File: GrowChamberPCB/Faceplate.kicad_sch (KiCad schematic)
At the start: 56 parts, among them J1 Mister, J10 FoggerBasin, J12 Moisture Sensor 3, J13 Moisture Sensor 2, J14 UART, J15 FAE Fan, J16 DrainLevel, J2 Moisture Sensor 1, J3 SCD30, J4 Heater Fans, J49 TP, J5 Fogger Solenoid, J50 TP, J6 Drain Solenoid, J7 Water Solenoid, J8 Glycol Solenoid, J9 CircFan, SW2 ResetButton_External, SW4 BootMode_External, U2 ZX-IDC2.54-2-13PZZ, U20 PCA9555APW,118

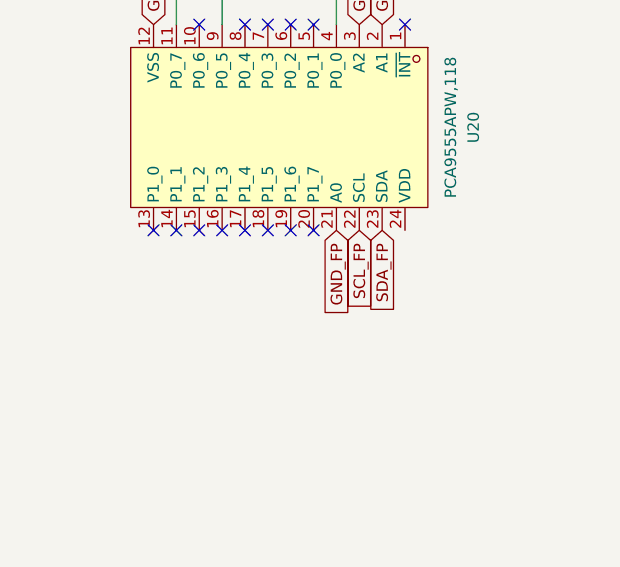
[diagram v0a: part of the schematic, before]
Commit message: working on pcb
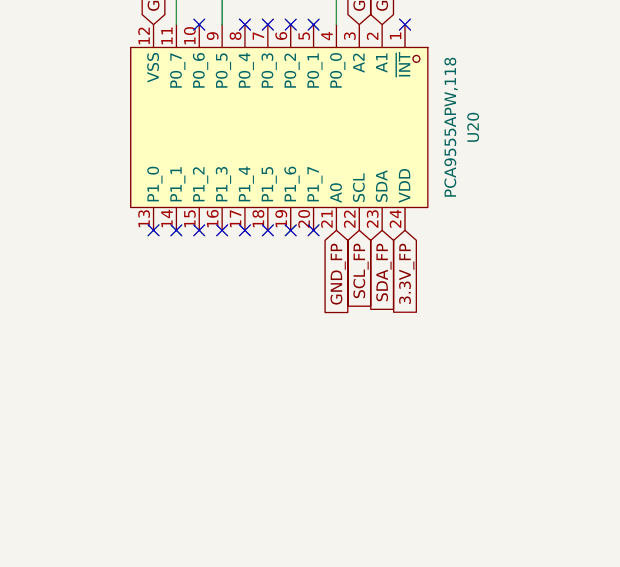
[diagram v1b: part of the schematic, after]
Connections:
- net 3.3V_FP: now also U20.24 (VDD)
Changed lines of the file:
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@@
+		)
+	)
+	(global_label "3.3V_FP"
+		(shape input)
+		(at 265.43 139.7 270)
+		(fields_autoplaced yes)
+		(effects
+			(font
+				(size 1.27 1.27)
+			)
+			(justify right)
+		)
+		(property "Intersheetrefs" "${INTERSHEET_REFS}"
+			(at 265.43 150.1238 90)
+			(hide yes)
+			(show_name no)
+			(do_not_autoplace no)
+			(effects
+				(font
+					(size 1.27 1.27)
+				)
+				(justify right)
+			)
 		)
 	)
